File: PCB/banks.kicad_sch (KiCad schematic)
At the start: 50 parts, among them U1 XC7A50T-FGG484, Y3 100MHz

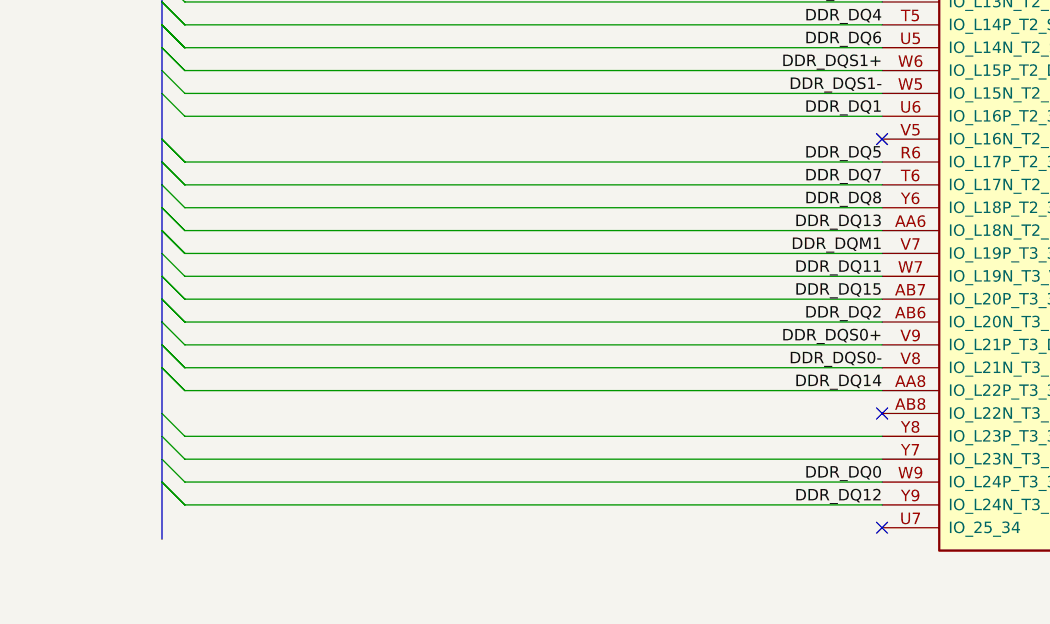
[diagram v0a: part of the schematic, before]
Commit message: KFNESIFHESKJFHSEKJFH UI DID IT
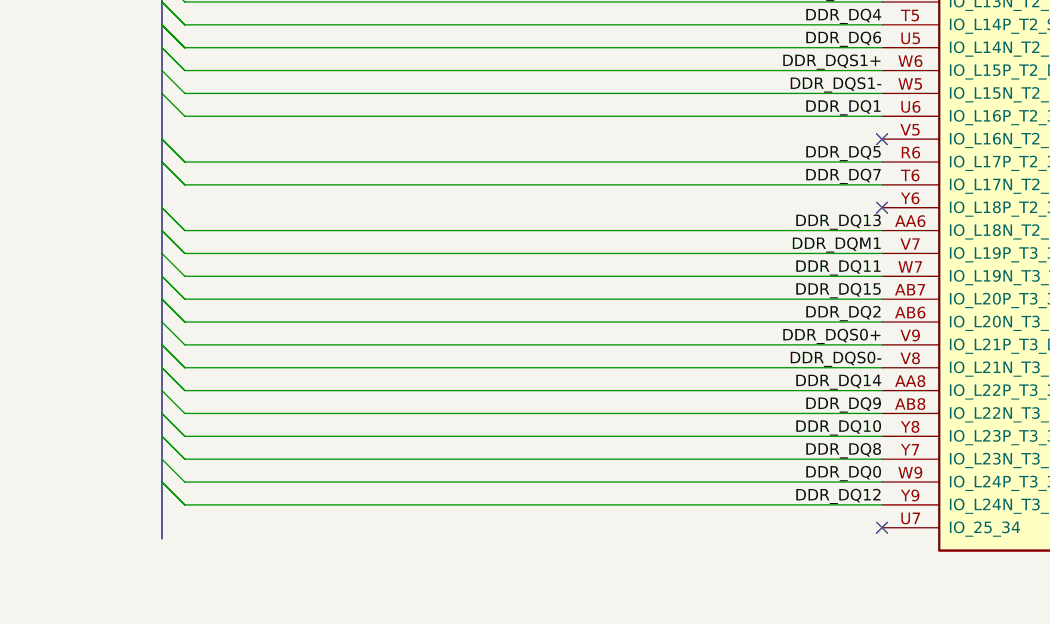
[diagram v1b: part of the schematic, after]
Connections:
- net DDR_DQ8: now also U1.Y7 (IO_L23N_T3_34); no longer U1.Y6 (IO_L18P_T2_34)
- net DDR_DQ9: now reaches U1.AB8 (IO_L22N_T3_34)
- net DDR_DQ10: now reaches U1.Y8 (IO_L23P_T3_34)
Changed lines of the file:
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@@
 	)
 	(no_connect
+		(at 702.31 179.07)
+	)
+	(no_connect
 		(at 261.62 209.55)
 	)
@@
 	)
 	(no_connect
-		(at 702.31 201.93)
-	)
-	(no_connect
 		(at 127 105.41)
 	)
@@
 	)
 	(bus_entry
+		(at 622.3 201.93)
+		(size 2.54 2.54)
+		(stroke
+			(width 0)
+			(type default)
+		)
+	)
+	(bus_entry
+		(at 622.3 204.47)
+		(size 2.54 2.54)
+		(stroke
+			(width 0)
+			(type default)
+		)
+	)
+	(bus_entry
 		(at 622.3 173.99)
 		(size 2.54 2.54)
@@
 	)
 	(bus_entry
-		(at 622.3 176.53)
-		(size 2.54 2.54)
+		(at 142.24 100.33)
+		(size 2.54 -2.54)
 		(stroke
 			(width 0)
@@
 	)
 	(bus_entry
-		(at 142.24 100.33)
-		(size 2.54 -2.54)
+		(at 622.3 199.39)
+		(size 2.54 2.54)
 		(stroke
 			(width 0)
@@
 		)
 	)
+	(bus
+		(pts
+			(xy 622.3 199.39) (xy 622.3 201.93)
+		)
+		(stroke
+			(width 0)
+			(type default)
+		)
+	)
 	(wire
 		(pts
@@
 	(wire
 		(pts
+			(xy 624.84 201.93) (xy 702.31 201.93)
+		)
+		(stroke
+			(width 0)
+			(type default)
+		)
+	)
+	(wire
+		(pts
 			(xy 154.94 149.86) (xy 146.05 149.86)
 		)
@@
 	(bus
 		(pts
-			(xy 622.3 196.85) (xy 622.3 201.93)
+			(xy 622.3 196.85) (xy 622.3 199.39)
 		)
 		(stroke
@@
 	(wire
 		(pts
-			(xy 624.84 204.47) (xy 702.31 204.47)
+			(xy 300.99 49.53) (xy 308.61 49.53)
 		)
 		(stroke
@@
 	(wire
 		(pts
-			(xy 300.99 49.53) (xy 308.61 49.53)
+			(xy 624.84 186.69) (xy 702.31 186.69)
 		)
 		(stroke
@@
 	(wire
 		(pts
-			(xy 624.84 186.69) (xy 702.31 186.69)
+			(xy 300.99 62.23) (xy 300.99 59.69)
 		)
 		(stroke
@@
 		)
 	)
-	(wire
+	(bus
 		(pts
-			(xy 300.99 62.23) (xy 300.99 59.69)
+			(xy 182.88 154.94) (xy 179.07 154.94)
 		)
 		(stroke
@@
 		)
 	)
-	(bus
+	(wire
 		(pts
-			(xy 182.88 154.94) (xy 179.07 154.94)
+			(xy 361.95 49.53) (xy 361.95 52.07)
 		)
 		(stroke
@@
 	(wire
 		(pts
-			(xy 361.95 49.53) (xy 361.95 52.07)
+			(xy 624.84 207.01) (xy 702.31 207.01)
 		)
 		(stroke
@@
 		)
 	)
-	(bus
-		(pts
-			(xy 622.3 173.99) (xy 622.3 176.53)
-		)
-		(stroke
-			(width 0)
-			(type default)
-		)
-	)
 	(wire
 		(pts
@@
 	(wire
 		(pts
-			(xy 624.84 179.07) (xy 702.31 179.07)
-		)
-		(stroke
-			(width 0)
-			(type default)
-		)
-	)
-	(wire
-		(pts
 			(xy 146.05 149.86) (xy 146.05 151.13)
 		)
@@
 	(bus
 		(pts
-			(xy 622.3 176.53) (xy 622.3 179.07)
+			(xy 622.3 173.99) (xy 622.3 179.07)
 		)
 		(stroke
@@
 	(wire
 		(pts
-			(xy 624.84 207.01) (xy 702.31 207.01)
-		)
-		(stroke
-			(width 0)
-			(type default)
-		)
-	)
-	(wire
-		(pts
 			(xy 154.94 158.75) (xy 154.94 163.83)
 		)
@@
 	(wire
 		(pts
+			(xy 624.84 204.47) (xy 702.31 204.47)
+		)
+		(stroke
+			(width 0)
+			(type default)
+		)
+	)
+	(wire
+		(pts
 			(xy 285.75 62.23) (xy 285.75 59.69)
 		)
@@
 		)
 	)
-	(label "DDR_DQ8"
-		(at 702.31 179.07 180)
-		(effects
-			(font
-				(size 1.27 1.27)
-			)
-			(justify right bottom)
-		)
-	)
 	(label "DDR_A11"
 		(at 702.31 115.57 180)
@@
 		)
 	)
+	(label "DDR_DQ8"
+		(at 702.31 207.01 180)
+		(effects
+			(font
+				(size 1.27 1.27)
+			)
+			(justify right bottom)
+		)
+	)
 	(label "DDR_DQ4"
 		(at 702.31 158.75 180)
@@
 		)
 	)
+	(label "DDR_DQ10"
+		(at 702.31 204.47 180)
+		(effects
+			(font
+				(size 1.27 1.27)
+			)
+			(justify right bottom)
+		)
+	)
 	(label "DDR_DQ11"
 		(at 702.31 186.69 180)
@@
 		(effects
 			(font
+				(size 1.27 1.27)
+			)
+			(justify right bottom)
+		)
+	)
+	(label "DDR_DQ9"
+		(at 702.31 201.93 180)
+		(effects
+			(font
